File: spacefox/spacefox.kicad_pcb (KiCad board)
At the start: 2 copper layers, 100 x 87 mm, 7 parts, among them U1 ProMicro

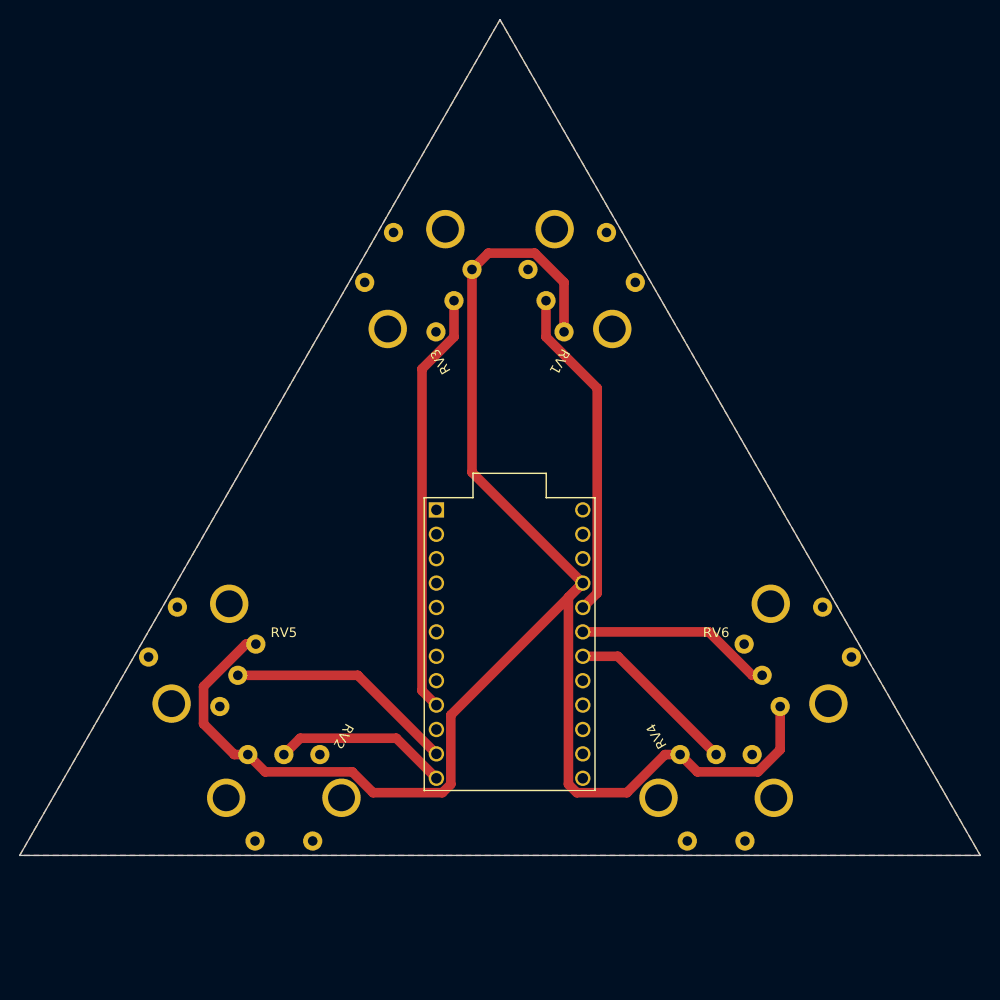
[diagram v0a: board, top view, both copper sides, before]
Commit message: WIP V2 PCB
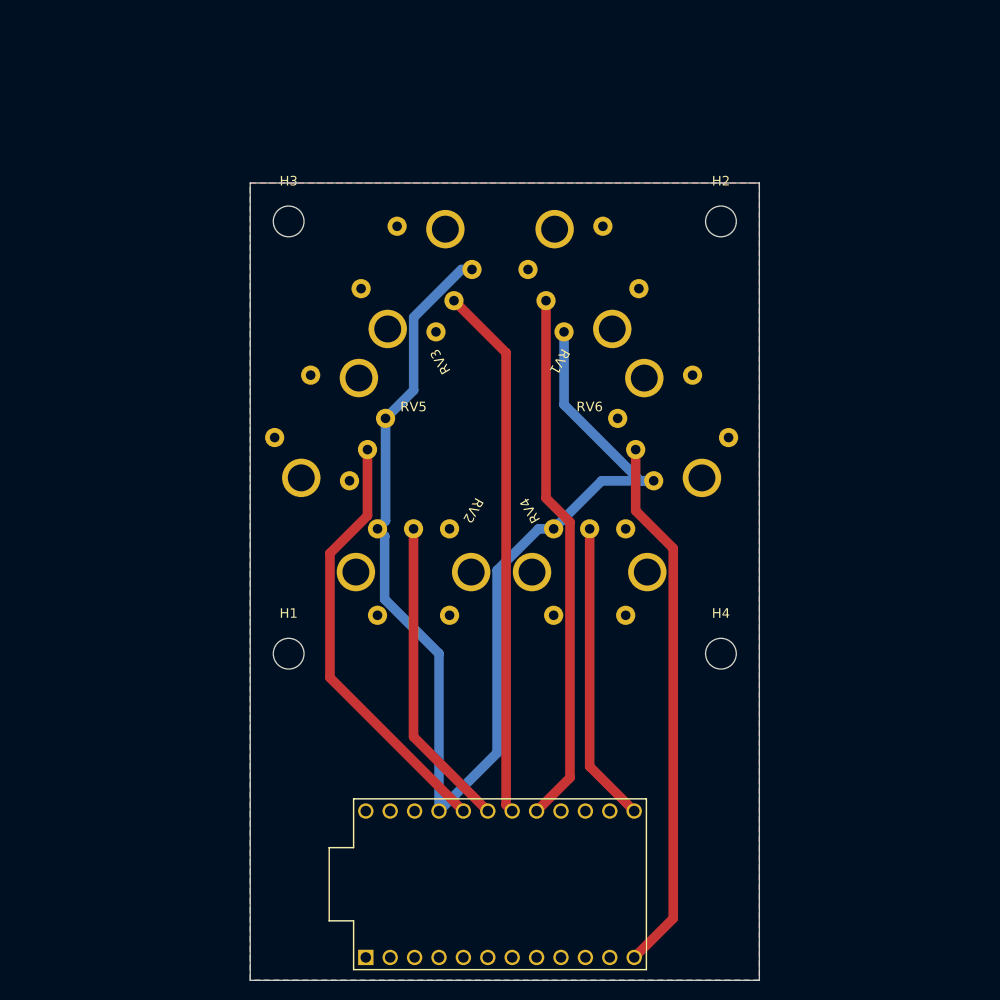
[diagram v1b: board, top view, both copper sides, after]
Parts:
- added H1: MountingHole, MountingHole:MountingHole_3.2mm_M3, F.Cu at (133.0, 99.0)
- added H2: MountingHole, MountingHole:MountingHole_3.2mm_M3, F.Cu at (178.0, 54.0)
- added H3: MountingHole, MountingHole:MountingHole_3.2mm_M3, F.Cu at (133.0, 54.0)
- added H4: MountingHole, MountingHole:MountingHole_3.2mm_M3, F.Cu at (178.0, 99.0)
- moved RV2 27.1 mm to (141.2, 77.8)
- moved RV5 27.1 mm to (146.0, 86.0)
- moved RV4 26.9 mm to (169.1, 77.8)
- moved RV6 26.9 mm to (164.3, 86.0)
- moved U1 25.0 mm to (155.0, 123.0), turned to 0 degrees
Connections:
- RV2 pad 2: Net-(RV2-Pad2) -> Net-(U1-Pad20)
- RV3 pad 2: Net-(U1-Pad20) -> Net-(RV3-Pad2)
- RV4 pad 2: Net-(U1-Pad19) -> Net-(U1-Pad12)
- RV6 pad 2: Net-(RV6-Pad2) -> Net-(U1-Pad13)
- U1 pad 11: Net-(RV2-Pad2) -> unconnected-(U1-Pad11)
- U1 pad 12: Net-(RV5-Pad2) -> Net-(U1-Pad12)
- U1 pad 13: unconnected-(U1-Pad13) -> Net-(U1-Pad13)
- U1 pad 17: unconnected-(U1-Pad17) -> Net-(RV3-Pad2)
- U1 pad 18: Net-(RV6-Pad2) -> Net-(RV1-Pad2)
- U1 pad 19: Net-(U1-Pad19) -> Net-(RV5-Pad2)
- U1 pad 9: Net-(RV1-Pad2) -> unconnected-(U1-Pad9)
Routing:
- net Net-(U1-Pad12): track 0.00 -> 56.2 mm
- net Net-(RV3-Pad2): track 0.00 -> 55.6 mm
- net VCC: track 172.8 -> 131.7 mm
- net Net-(U1-Pad13): track 0.00 -> 31.3 mm
- net Net-(RV2-Pad2): track 24.1 -> 0.00 mm
- net Net-(U1-Pad19): track 20.5 -> 0.00 mm
- net Net-(RV6-Pad2): track 18.1 -> 0.00 mm
- net Net-(RV5-Pad2): track 18.3 -> 32.6 mm
- net Net-(RV1-Pad2): track 44.1 -> 55.6 mm
- net Net-(U1-Pad20): track 34.8 -> 45.0 mm
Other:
- board size 100 x 87 mm -> 53 x 83 mm
